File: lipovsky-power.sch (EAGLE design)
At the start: 99 parts, among them Q11 NMOS40V_10A, Q12 NMOS40V_10A, Q14 NMOS40V_10A, Q15 NMOS40V_10A, Q16 NMOS40V_10A, Q18 NMOS40V_10A, Q2 2NMOS30V_0.1A, Q21 PMOS30V_11A, Q22 PMOS30V_11A, Q23 NMOS40V_10A, Q24 NMOS40V_10A, Q25 PMOS30V_11A, Q26 PMOS30V_11A, Q27 NMOS40V_10A, Q28 NMOS40V_10A, Q3 2PMOS50V_0.17A, Q31 PMOS30V_11A, Q32 PMOS30V_11A, Q33 PMOS30V_11A, Q34 PMOS30V_11A, Q35 PMOS30V_11A, Q36 PMOS30V_11A, Q37 PMOS30V_11A, Q38 PMOS30V_11A, Q4 2PMOS50V_0.17A, Q41 PMOS30V_11A, Q42 PMOS30V_11A, Q43 PMOS30V_11A, Q44 PMOS30V_11A, Q45 PMOS30V_11A, Q46 PMOS30V_11A, Q47 PMOS30V_11A, Q48 PMOS30V_11A, Q5 2NMOS30V_0.1A, Q51 PMOS30V_11A, Q52 PMOS30V_11A, Q53 PMOS30V_11A, Q54 PMOS30V_11A, Q55 PMOS30V_11A, Q56 PMOS30V_11A, Q57 PMOS30V_11A, Q58 PMOS30V_11A, Q62 PMOS30V_11A, Q64 PMOS30V_11A, Q66 PMOS30V_11A, Q68 PMOS30V_11A, T1 TFORM_4_4311_4A4, U1 DG508BEN-T1-GE4, U2 DG508BEN-T1-GE4, U3 74HC595, U4 LTC3805-5IDD, U5 TC1240A, U6 AR30N60PPA-13

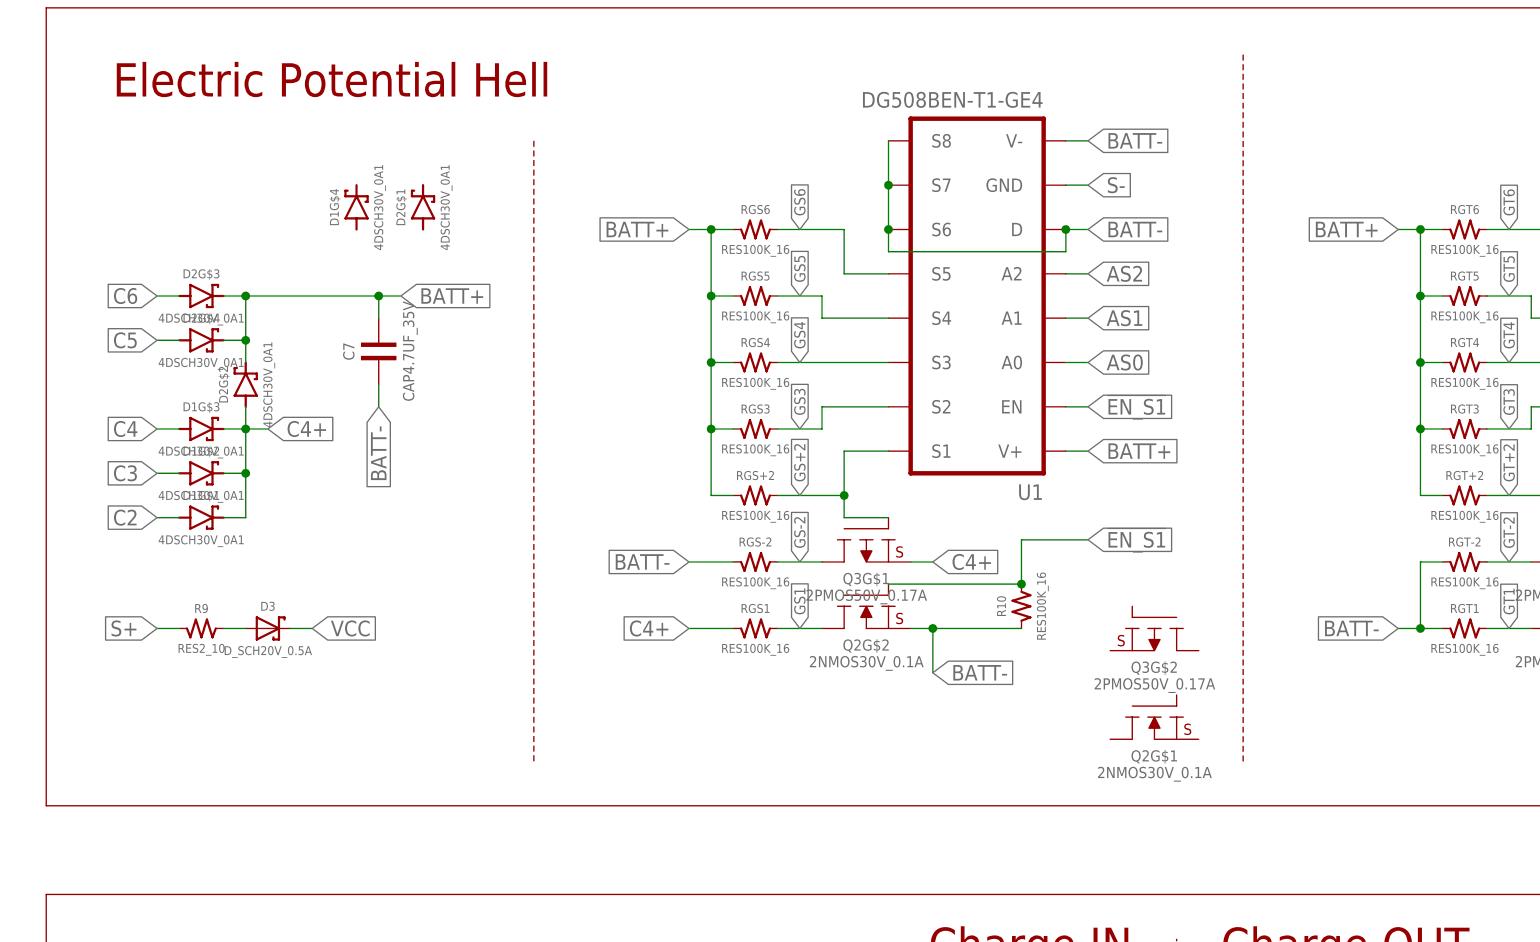
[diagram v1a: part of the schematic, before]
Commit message: laying out
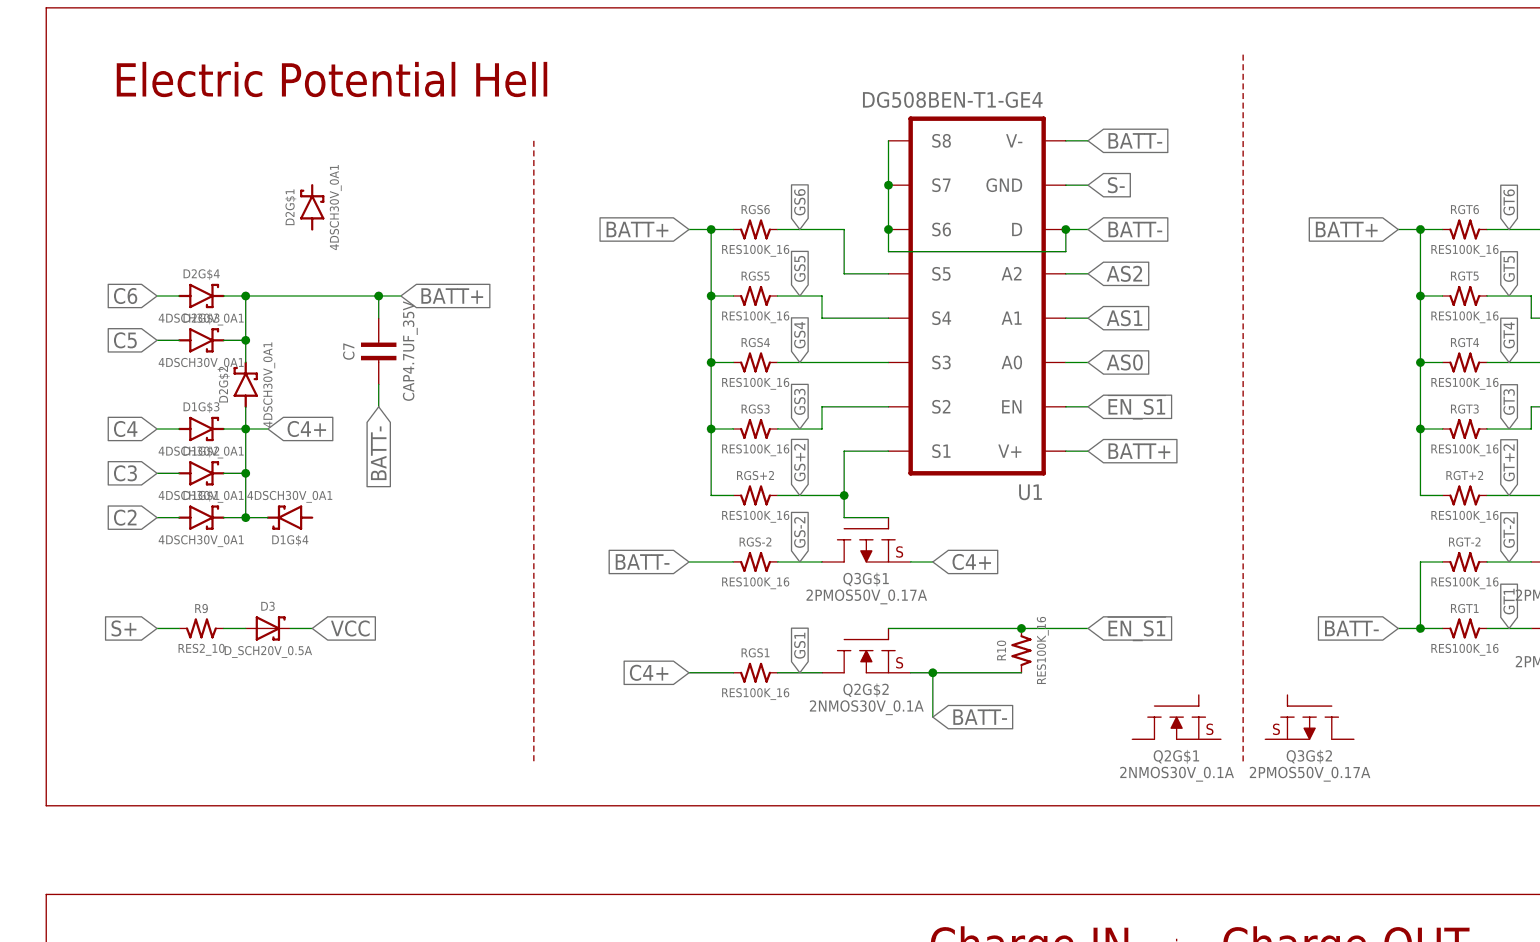
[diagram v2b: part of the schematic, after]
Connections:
- net C4+: now also D1G$4.C
- net C5: now also D2G$3.A; no longer D2G$4.A
- net C6: now also D2G$4.A; no longer D2G$3.A
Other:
- moved on the sheet: D1G$4, D2G$1, D2G$3, D2G$4, Q2G$1, Q2G$2, Q3G$2, R10, RGS1
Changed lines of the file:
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@@
 <instance part="D1" gate="G$2" x="22.86" y="43.18"/>
 <instance part="D1" gate="G$3" x="22.86" y="48.26"/>
-<instance part="D1" gate="G$4" x="40.64" y="73.66" rot="R90"/>
-<instance part="D2" gate="G$3" x="22.86" y="63.5"/>
+<instance part="D1" gate="G$4" x="33.02" y="38.1" rot="R180"/>
+<instance part="D2" gate="G$3" x="22.86" y="58.42"/>
 <instance part="R1" gate="G$1" x="-76.2" y="-48.26" rot="R90"/>
 <instance part="R2" gate="G$1" x="-20.32" y="-48.26" rot="R90"/>
@@
 <instance part="Q23" gate="G$1" x="-101.6" y="-35.56" rot="MR270"/>
 <instance part="Q24" gate="G$1" x="-86.36" y="-35.56" rot="R270"/>
-<instance part="RGS1" gate="G$1" x="86.36" y="25.4"/>
-<instance part="D2" gate="G$4" x="22.86" y="58.42"/>
+<instance part="RGS1" gate="G$1" x="86.36" y="20.32"/>
+<instance part="D2" gate="G$4" x="22.86" y="63.5"/>
 <instance part="RGS-2" gate="G$1" x="86.36" y="33.02"/>
-<instance part="Q2" gate="G$2" x="99.06" y="25.4" rot="MR270"/>
+<instance part="Q2" gate="G$2" x="99.06" y="20.32" rot="MR270"/>
 <instance part="Q27" gate="G$1" x="-45.72" y="-35.56" rot="MR270"/>
 <instance part="Q28" gate="G$1" x="-30.48" y="-35.56" rot="R270"/>
@@
 <instance part="R9" gate="G$1" x="22.86" y="25.4"/>
 <instance part="D3" gate="G$1" x="30.48" y="25.4"/>
-<instance part="R10" gate="G$1" x="116.84" y="27.94" rot="R90"/>
+<instance part="R10" gate="G$1" x="116.84" y="22.86" rot="R90"/>
 <instance part="C3" gate="G$1" x="43.18" y="-27.94" rot="R90"/>
 <instance part="C7" gate="G$1" x="43.18" y="55.88" rot="R90"/>
@@
 <instance part="R15" gate="G$1" x="167.64" y="-45.72"/>
 <instance part="C10" gate="G$1" x="160.02" y="-33.02" rot="R90"/>
-<instance part="Q2" gate="G$1" x="132.08" y="12.7" rot="MR270"/>
+<instance part="Q2" gate="G$1" x="134.62" y="12.7" rot="MR270"/>
 <instance part="R17" gate="G$1" x="144.78" y="-53.34" rot="R90"/>
 <instance part="R18" gate="G$1" x="152.4" y="-63.5" rot="R180"/>
 <instance part="Q5" gate="G$1" x="119.38" y="-55.88"/>
 <instance part="Q5" gate="G$2" x="152.4" y="-68.58" rot="R90"/>
-<instance part="Q3" gate="G$2" x="132.08" y="22.86" rot="R270"/>
-<instance part="D2" gate="G$1" x="48.26" y="73.66" rot="R90"/>
+<instance part="Q3" gate="G$2" x="149.86" y="12.7" rot="R270"/>
+<instance part="D2" gate="G$1" x="35.56" y="73.66" rot="R90"/>
 <instance part="D2" gate="G$2" x="27.94" y="53.34" rot="R90"/>
 </instances>
@@
 </segment>
 <segment>
-<wire x1="20.32" y1="48.26" x2="17.78" y2="48.26" width="0.1524" layer="91"/>
 <label x="17.78" y="48.26" size="1.778" layer="95" rot="R180" xref="yes"/>
 <pinref part="D1" gate="G$3" pin="A"/>
+<wire x1="17.78" y1="48.26" x2="20.32" y2="48.26" width="0.1524" layer="91"/>
 </segment>
 <segment>
@@
 <segment>
 <label x="17.78" y="58.42" size="1.778" layer="95" rot="R180" xref="yes"/>
-<pinref part="D2" gate="G$4" pin="A"/>
+<pinref part="D2" gate="G$3" pin="A"/>
 <wire x1="17.78" y1="58.42" x2="20.32" y2="58.42" width="0.1524" layer="91"/>
 </segment>
@@
 </segment>
 <segment>
-<pinref part="D2" gate="G$3" pin="A"/>
-<wire x1="20.32" y1="63.5" x2="17.78" y2="63.5" width="0.1524" layer="91"/>
 <label x="17.78" y="63.5" size="1.778" layer="95" rot="R180" xref="yes"/>
+<pinref part="D2" gate="G$4" pin="A"/>
+<wire x1="17.78" y1="63.5" x2="20.32" y2="63.5" width="0.1524" layer="91"/>
 </segment>
 </net>
@@
 <segment>
 <pinref part="Q2" gate="G$2" pin="S"/>
-<wire x1="104.14" y1="25.4" x2="106.68" y2="25.4" width="0.1524" layer="91"/>
-<wire x1="106.68" y1="25.4" x2="106.68" y2="20.32" width="0.1524" layer="91"/>
-<label x="106.68" y="20.32" size="1.778" layer="95" xref="yes"/>
+<wire x1="104.14" y1="20.32" x2="106.68" y2="20.32" width="0.1524" layer="91"/>
+<wire x1="106.68" y1="20.32" x2="106.68" y2="15.24" width="0.1524" layer="91"/>
+<label x="106.68" y="15.24" size="1.778" layer="95" xref="yes"/>
 <pinref part="R10" gate="G$1" pin="1"/>
-<wire x1="106.68" y1="25.4" x2="116.84" y2="25.4" width="0.1524" layer="91"/>
-<junction x="106.68" y="25.4"/>
+<wire x1="106.68" y1="20.32" x2="116.84" y2="20.32" width="0.1524" layer="91"/>
+<junction x="106.68" y="20.32"/>
 </segment>
 <segment>
@@
 <segment>
 <pinref part="RGS1" gate="G$1" pin="2"/>
-<wire x1="88.9" y1="25.4" x2="93.98" y2="25.4" width="0.1524" layer="91"/>
-<label x="91.44" y="25.4" size="1.27" layer="95" rot="R90" xref="yes"/>
+<wire x1="88.9" y1="20.32" x2="93.98" y2="20.32" width="0.1524" layer="91"/>
+<label x="91.44" y="20.32" size="1.27" layer="95" rot="R90" xref="yes"/>
 <pinref part="Q2" gate="G$2" pin="D"/>
 </segment>
@@
 </segment>
 <segment>
-<pinref part="D2" gate="G$4" pin="C"/>
-<pinref part="D2" gate="G$3" pin="C"/>
-<wire x1="27.94" y1="63.5" x2="25.4" y2="63.5" width="0.1524" layer="91"/>
-<junction x="27.94" y="63.5"/>
 <wire x1="27.94" y1="63.5" x2="43.18" y2="63.5" width="0.1524" layer="91"/>
 <wire x1="43.18" y1="63.5" x2="45.72" y2="63.5" width="0.1524" layer="91"/>
 <wire x1="27.94" y1="63.5" x2="27.94" y2="58.42" width="0.1524" layer="91"/>
-<wire x1="27.94" y1="58.42" x2="25.4" y2="58.42" width="0.1524" layer="91"/>
 <label x="45.72" y="63.5" size="1.778" layer="95" xref="yes"/>
 <pinref part="C7" gate="G$1" pin="2"/>
 <wire x1="43.18" y1="63.5" x2="43.18" y2="60.96" width="0.1524" layer="91"/>
 <junction x="43.18" y="63.5"/>
+<pinref part="D2" gate="G$3" pin="C"/>
+<wire x1="27.94" y1="58.42" x2="25.4" y2="58.42" width="0.1524" layer="91"/>
+<pinref part="D2" gate="G$4" pin="C"/>
+<wire x1="27.94" y1="63.5" x2="25.4" y2="63.5" width="0.1524" layer="91"/>
+<junction x="27.94" y="63.5"/>
 <pinref part="D2" gate="G$2" pin="C"/>
-<wire x1="27.94" y1="55.88" x2="27.94" y2="58.42" width="0.1524" layer="91"/>
+<wire x1="27.94" y1="58.42" x2="27.94" y2="55.88" width="0.1524" layer="91"/>
 <junction x="27.94" y="58.42"/>
 </segment>
@@
 <net name="C4+" class="0">
 <segment>
-<pinref part="D1" gate="G$3" pin="C"/>
-<wire x1="25.4" y1="48.26" x2="27.94" y2="48.26" width="0.1524" layer="91"/>
 <wire x1="27.94" y1="48.26" x2="27.94" y2="43.18" width="0.1524" layer="91"/>
 <pinref part="D1" gate="G$2" pin="C"/>
@@
 <wire x1="27.94" y1="48.26" x2="30.48" y2="48.26" width="0.1524" layer="91"/>
 <label x="30.48" y="48.26" size="1.778" layer="95" xref="yes"/>
+<pinref part="D1" gate="G$3" pin="C"/>
+<wire x1="27.94" y1="48.26" x2="25.4" y2="48.26" width="0.1524" layer="91"/>
+<pinref part="D1" gate="G$4" pin="C"/>
+<wire x1="27.94" y1="38.1" x2="30.48" y2="38.1" width="0.1524" layer="91"/>
+<junction x="27.94" y="38.1"/>
 <pinref part="D2" gate="G$2" pin="A"/>
-<wire x1="27.94" y1="50.8" x2="27.94" y2="48.26" width="0.1524" layer="91"/>
+<wire x1="27.94" y1="48.26" x2="27.94" y2="50.8" width="0.1524" layer="91"/>
 </segment>
 <segment>
 <pinref part="RGS1" gate="G$1" pin="1"/>
-<wire x1="83.82" y1="25.4" x2="78.74" y2="25.4" width="0.1524" layer="91"/>
-<label x="78.74" y="25.4" size="1.778" layer="95" rot="R180" xref="yes"/>
+<wire x1="83.82" y1="20.32" x2="78.74" y2="20.32" width="0.1524" layer="91"/>
+<label x="78.74" y="20.32" size="1.778" layer="95" rot="R180" xref="yes"/>
 </segment>
 <segment>
@@
 <segment>
 <pinref part="Q2" gate="G$2" pin="G"/>
-<wire x1="101.6" y1="30.48" x2="116.84" y2="30.48" width="0.1524" layer="91"/>
-<wire x1="116.84" y1="35.56" x2="124.46" y2="35.56" width="0.1524" layer="91"/>
-<label x="124.46" y="35.56" size="1.778" layer="95" xref="yes"/>
+<wire x1="101.6" y1="25.4" x2="116.84" y2="25.4" width="0.1524" layer="91"/>
+<wire x1="116.84" y1="25.4" x2="124.46" y2="25.4" width="0.1524" layer="91"/>
+<label x="124.46" y="25.4" size="1.778" layer="95" xref="yes"/>
 <pinref part="R10" gate="G$1" pin="2"/>
-<wire x1="116.84" y1="35.56" x2="116.84" y2="30.48" width="0.1524" layer="91"/>
-<junction x="116.84" y="30.48"/>
-</segment>
-<segment>
+<junction x="116.84" y="25.4"/>
+</segment>
+<segment>
